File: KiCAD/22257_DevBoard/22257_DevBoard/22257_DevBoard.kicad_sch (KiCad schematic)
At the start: 0 parts

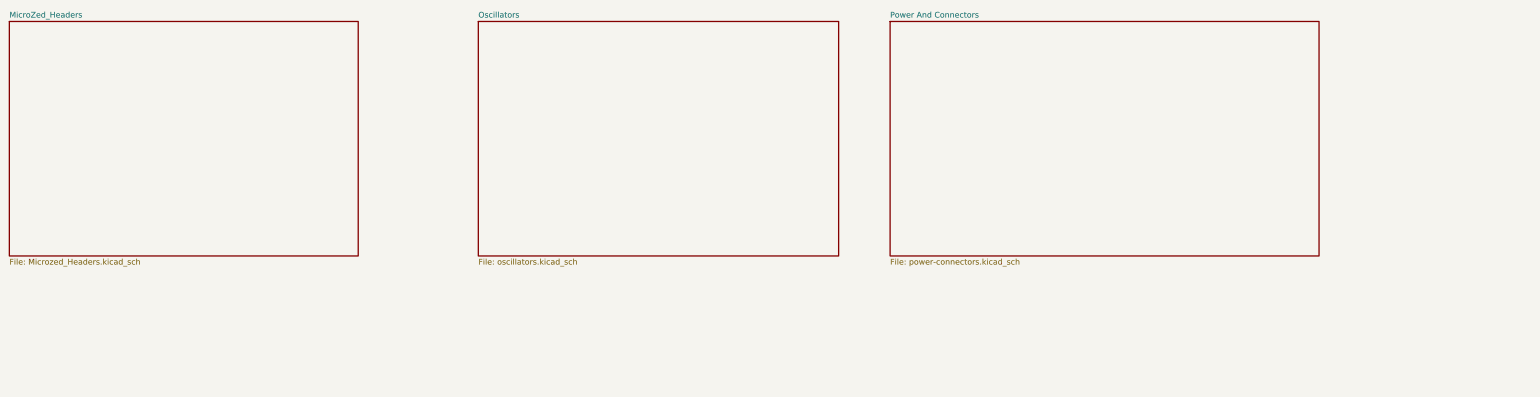
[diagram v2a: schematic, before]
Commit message: Done :D
Existence is pain
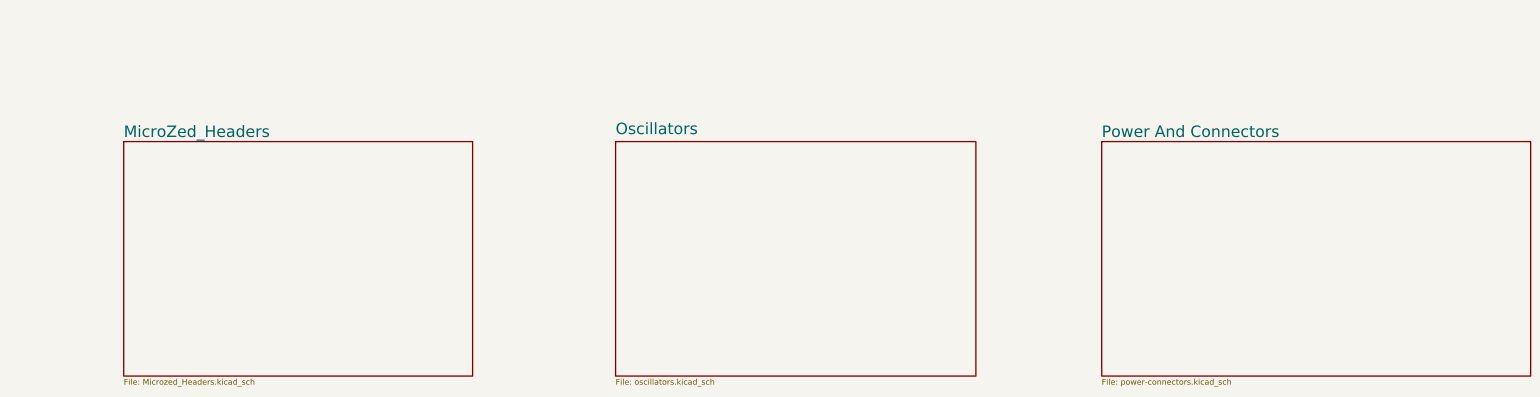
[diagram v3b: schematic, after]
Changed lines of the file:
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@@
 	(paper "A3")
 	(image
-		(at 146.05 189.23)
+		(at 208.28 179.07)
 		(scale 0.724029)
 		(data "iVBORw0KGgoAAAANSUhEUgAABKcAAAK6CAYAAADsGD8CAAAAAXNSR0IArs4c6QAAAARnQU1BAACx"
@@
 			"AAAAAAAAAAAAAAAAAAAAAAAAAAAAAAAAAAAAAAAAAAAAAAAAAAAAAAAAAAAAAAAAAAAAAAAAAAAA"
 			"AAAAAAAAAAAAAAAAAAAAAAAAAAAAAAAAAAAAAAAAAAAAAAAAAAAAAAAAAAAAAAAAAAAAAAAAAAAA"
+			"AAAAAAAAAAAAAAAAAAAAAAAAAAAAAAAAAAAAAAAAAAAAAAAAAAAAAAAAAAAAAAAAAAAAAAAAAAAA"
+			"AAAAAAAAAAAAAAAAAAAAAAAAAAAAAAAAAAAAAAAAAAAAAAAAAAAAAAAAAAAAAAAAAAAAAAAAAAAA"
+			"AAAAAAAAAAAAAAAAAAAAAAAAAAAAAAAAAAAAAAAAAAAAAAAAAAAAAAAAAAAAAAAAAAAAAAAAAAAA"
+			"AAAAAAAAAAAAAAAAAAAAAAAAAAAAAAAAAAAAAAAAAAAAAAAAAAAAAAAAAAAAAAAAAAAAAAAAAAAA"
+			"AAAAAAAAAAAAAAAAAAAAAAAAAAAAAAAAAAAAAAAAAAAAAAAAAAAAAAAAAAAAAAAAAAAAAAAAAAAA"
+			"AAAAAAAAAAAAAAAAAAAAAAAAAAAAAAAAAAAAAAAAAAAAAAAAAAAAAAAAAAAAAAAAAAAAAAAAAAAA"
+			"AAAAAAAAAAAAAAAAAAAAAAAAAAAAAAAAAAAAAAAAAAAAAAAAAAAAAAAAAAAAAAAAAAAAAAAAAAAA"
+			"AAAAAAAAAAAAAAAAAAAAAAAAAAAAAAAAAAAAAAAAAAAAAAAAAAAAAAAAAAAAAAAAAAAAAAAAAAAA"
+			"AAAAAAAAAAAAAAAAAAAAAAAAAAAAAAAAAAAAAAAAAAAAAAAAAAAAAAAAAAAAAAAAAAAAAAAAAAAA"
+			"AAAAAAAAAAAAAAAAAAAAAAAAAAAAAAAAAAAAAAAAAAAAAAAAAAAAAAAAAAAAAAAAAAAAAAAAAAAA"
+			"AAAAAAAAAAAAAAAAAAAAAAAAAAAAAAAAAAAAAAAAAAAAAAAAAAAAAAAAAAAAAAAAAAAAAAAAAAAA"
+			"AAAAAAAAAAAAAAAAAAAAAAAAAAAAAAAAAAAAAAAAAAAAAAAAAAAAAAAAAAAAAAAAAAAAAAAAAAAA"
+			"AAAAAAAAAAAAAAAAAAAAAAAAAAAAAAAAAAAAAAAAAAAAAAAAAAAAAAAAAAAAAAAAAAAAAAAAAAAA"
+			"AAAAAAAAAAAAAAAAAAAAAAAAAAAAAAAAAAAAAAAAAAAAAAAAAAAAAAAAAAAAAAAAAAAAAAAAAAAA"
+			"AAAAAAAAAAAAAAAAAAAAAAAAAAAAAAAAAAAAAAAAAAAAAAAAAAAAAAAAAAAAAAAAAAAAAAAAAAAA"
+			"AAAAAAAAAAAAAAAAAAAAAAAAAAAAAAAAAAAAAAAAAAAAAAAAAAAAAAAAAAAAAAAAAAAAAAAAAAAA"
+			"AAAAAAAAAAAAAAAAAAAAAAAAAAAAAAAAAAAAAAAAAAAAAAAAAAAAAAAAAAAAAAAAAAAAAAAAAAAA"
+			"AAAAAAAAAAAAAAAAAAAAAAAAAAAAAAAAAAAAAAAAAAAAAAAAAAAAAAAAAAAAAAAAAAAAAAAAAAAA"
 			"AAAAAAAAAAAAAAAAAAAAAAAAAA=="
 		)
 	)
 	(sheet
-		(at 219.71 19.05)
+		(at 266.7 45.72)
 		(size 95.25 52.07)
 		(exclude_from_sim no)
@@
 		)
 		(property "Sheetname" "Power And Connectors"
-			(at 219.71 18.3384 0)
+			(at 266.7 45.0084 0)
 			(effects
 				(font
-					(size 1.27 1.27)
+					(size 2.54 2.54)
 				)
 				(justify left bottom)
@@
 		)
 		(property "Sheetfile" "power-connectors.kicad_sch"
-			(at 219.71 71.7046 0)
+			(at 266.7 98.3746 0)
 			(effects
 				(font
@@
 	)
 	(sheet
-		(at 24.13 19.05)
+		(at 49.53 45.72)
 		(size 77.47 52.07)
 		(exclude_from_sim no)
@@
 		)
 		(property "Sheetname" "MicroZed_Headers"
-			(at 24.13 18.3384 0)
+			(at 49.53 45.0084 0)
 			(effects
 				(font
-					(size 1.27 1.27)
+					(size 2.54 2.54)
 				)
 				(justify left bottom)
@@
 		)
 		(property "Sheetfile" "Microzed_Headers.kicad_sch"
-			(at 24.13 71.7046 0)
+			(at 49.53 98.3746 0)
 			(effects
 				(font
@@
 	)
 	(sheet
-		(at 128.27 19.05)
+		(at 158.75 45.72)
 		(size 80.01 52.07)
 		(exclude_from_sim no)
@@
 		)
 		(property "Sheetname" "Oscillators"
-			(at 128.27 18.3384 0)
-			(show_name yes)
+			(at 158.75 44.3734 0)
 			(effects
 				(font
-					(size 1.27 1.27)
+					(size 2.54 2.54)
 				)
 				(justify left bottom)
@@
 		)
 		(property "Sheetfile" "oscillators.kicad_sch"
-			(at 128.27 71.7046 0)
+			(at 158.75 98.3746 0)
 			(effects
 				(font
